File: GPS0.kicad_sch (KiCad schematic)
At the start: 12 parts, among them J2 GPS_ANT_0, U2 MAX-M10S-00B

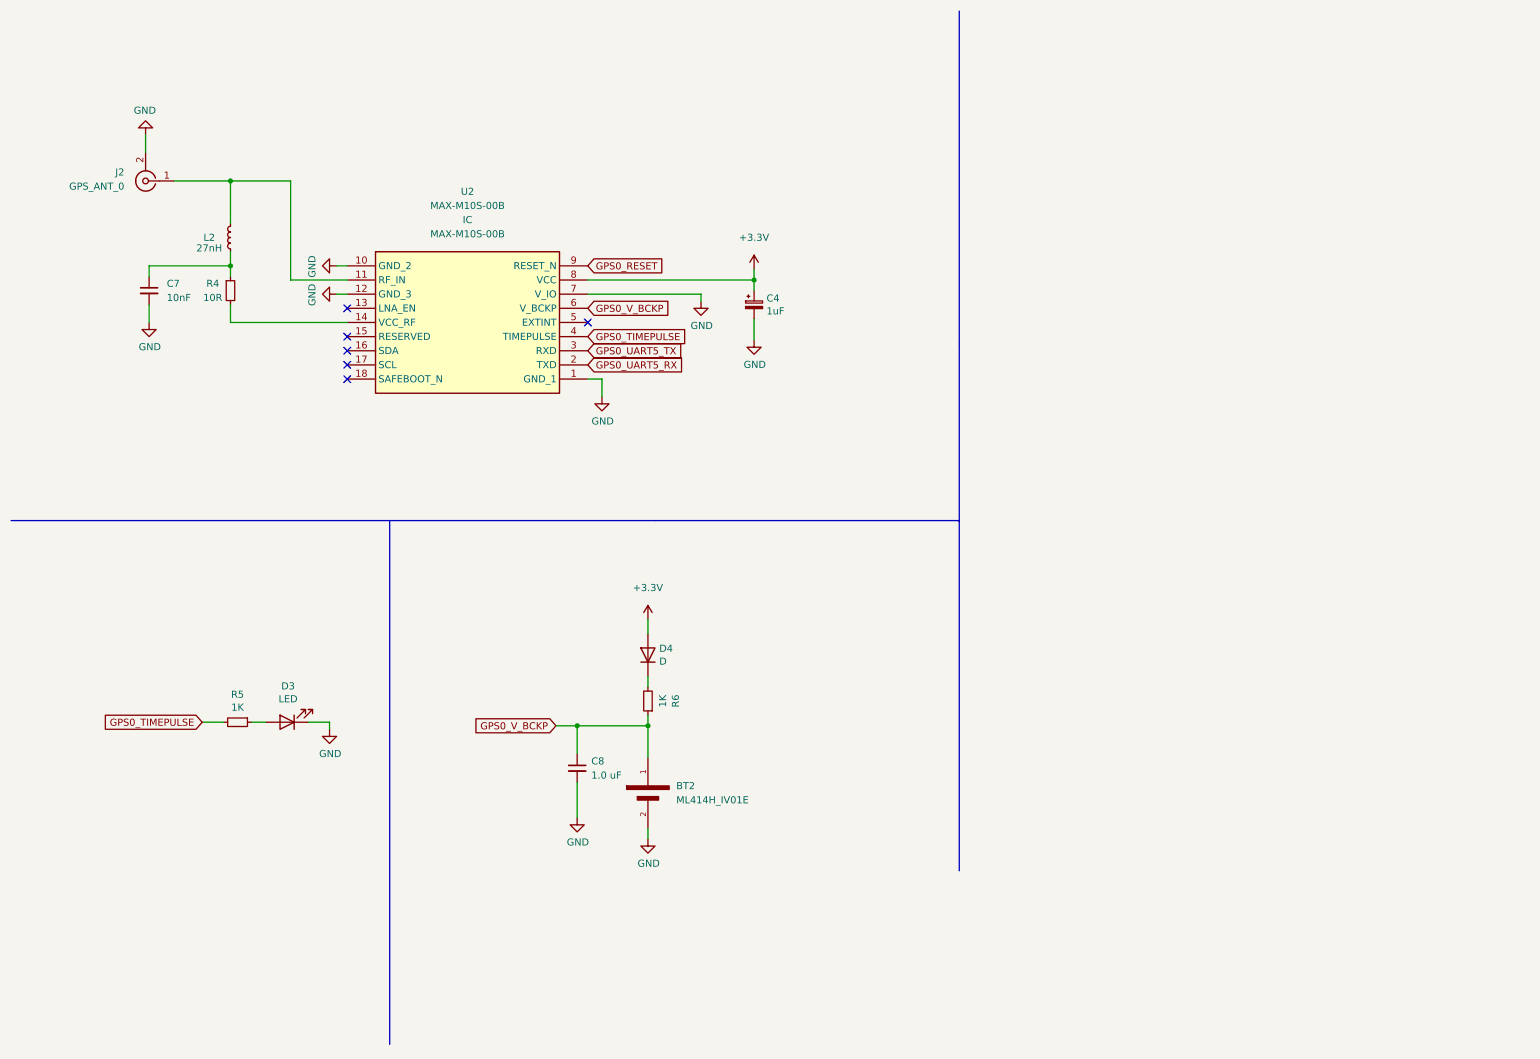
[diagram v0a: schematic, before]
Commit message: Last commit
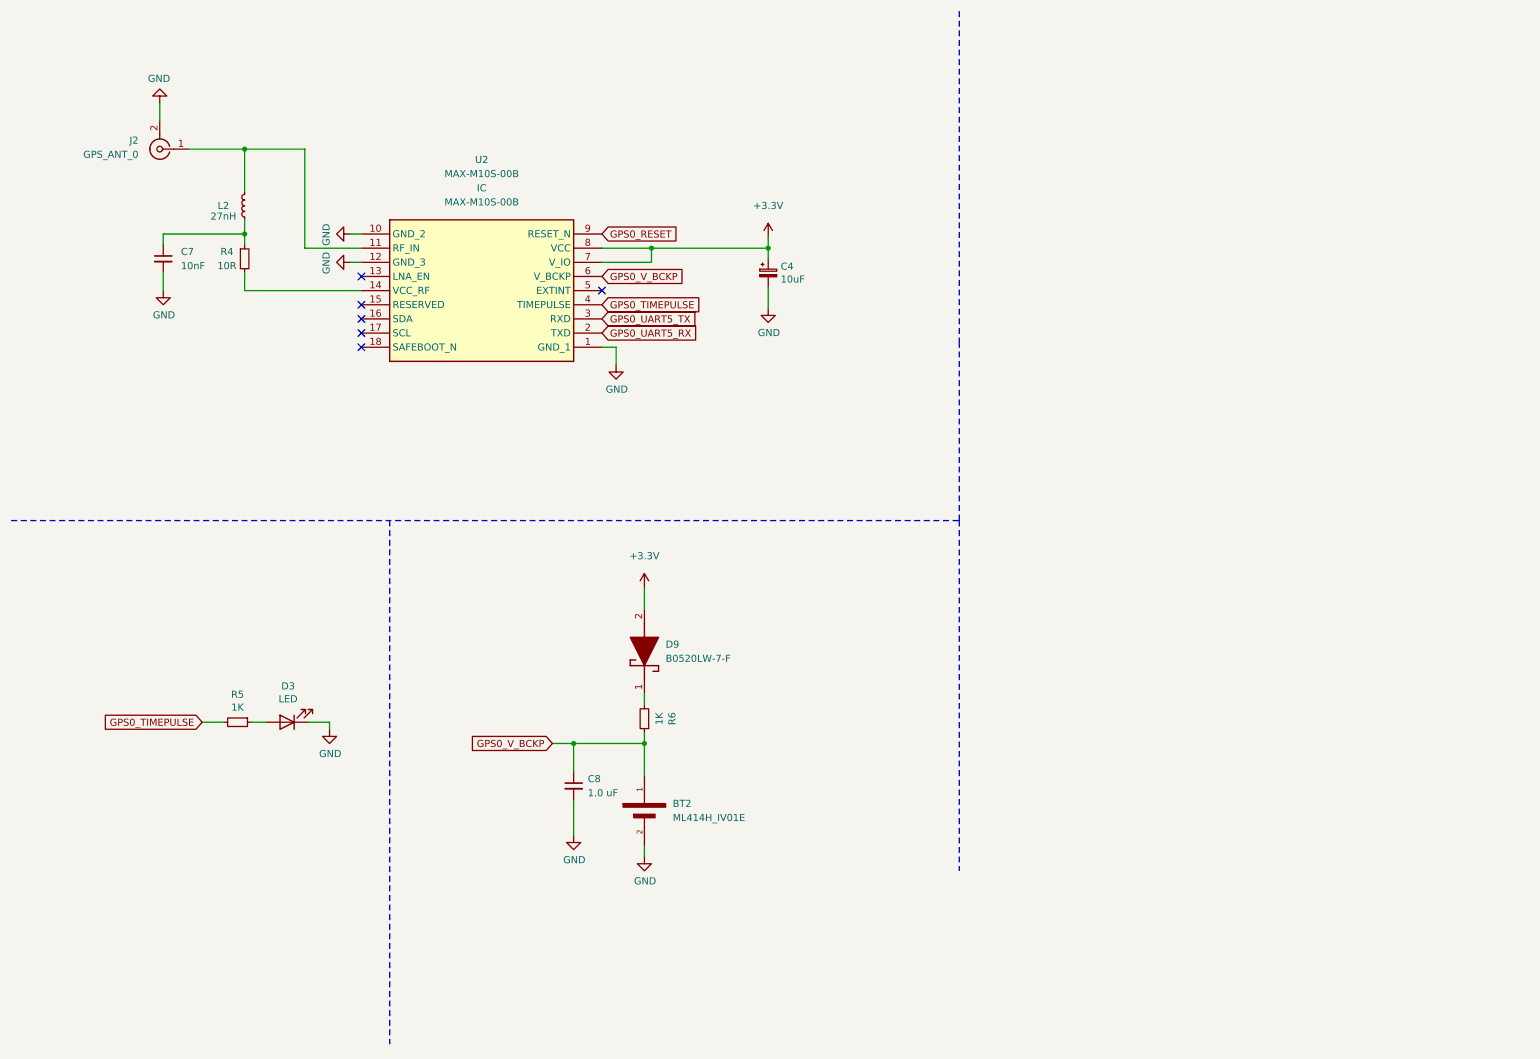
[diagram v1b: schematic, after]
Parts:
- removed D4: D, Diode_SMD:D_1206_3216Metric_Pad1.42x1.75mm_HandSolder, symbol Device:D
- added D9: B0520LW-7-F, B0520LW-7-F:SOD3716X145N, symbol B0520LW-7-F:B0520LW-7-F
- C4: value 1uF -> 10uF; footprint Capacitor_Tantalum_SMD:CP_EIA-3528-21_Kemet-B_Pad1.50x2.35mm_HandSolder -> Capacitor_SMD:C_1210_3225Metric
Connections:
- net +3.3V: now also U2.7 (V_IO), D9.2 (A)
- net GND: no longer U2.7 (V_IO)
- net at R6.2: now also D9.1 (K)
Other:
- moved on the sheet: BT2, C4, C7, C8, J2, L2, R4, R6, U2

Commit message: Second commit
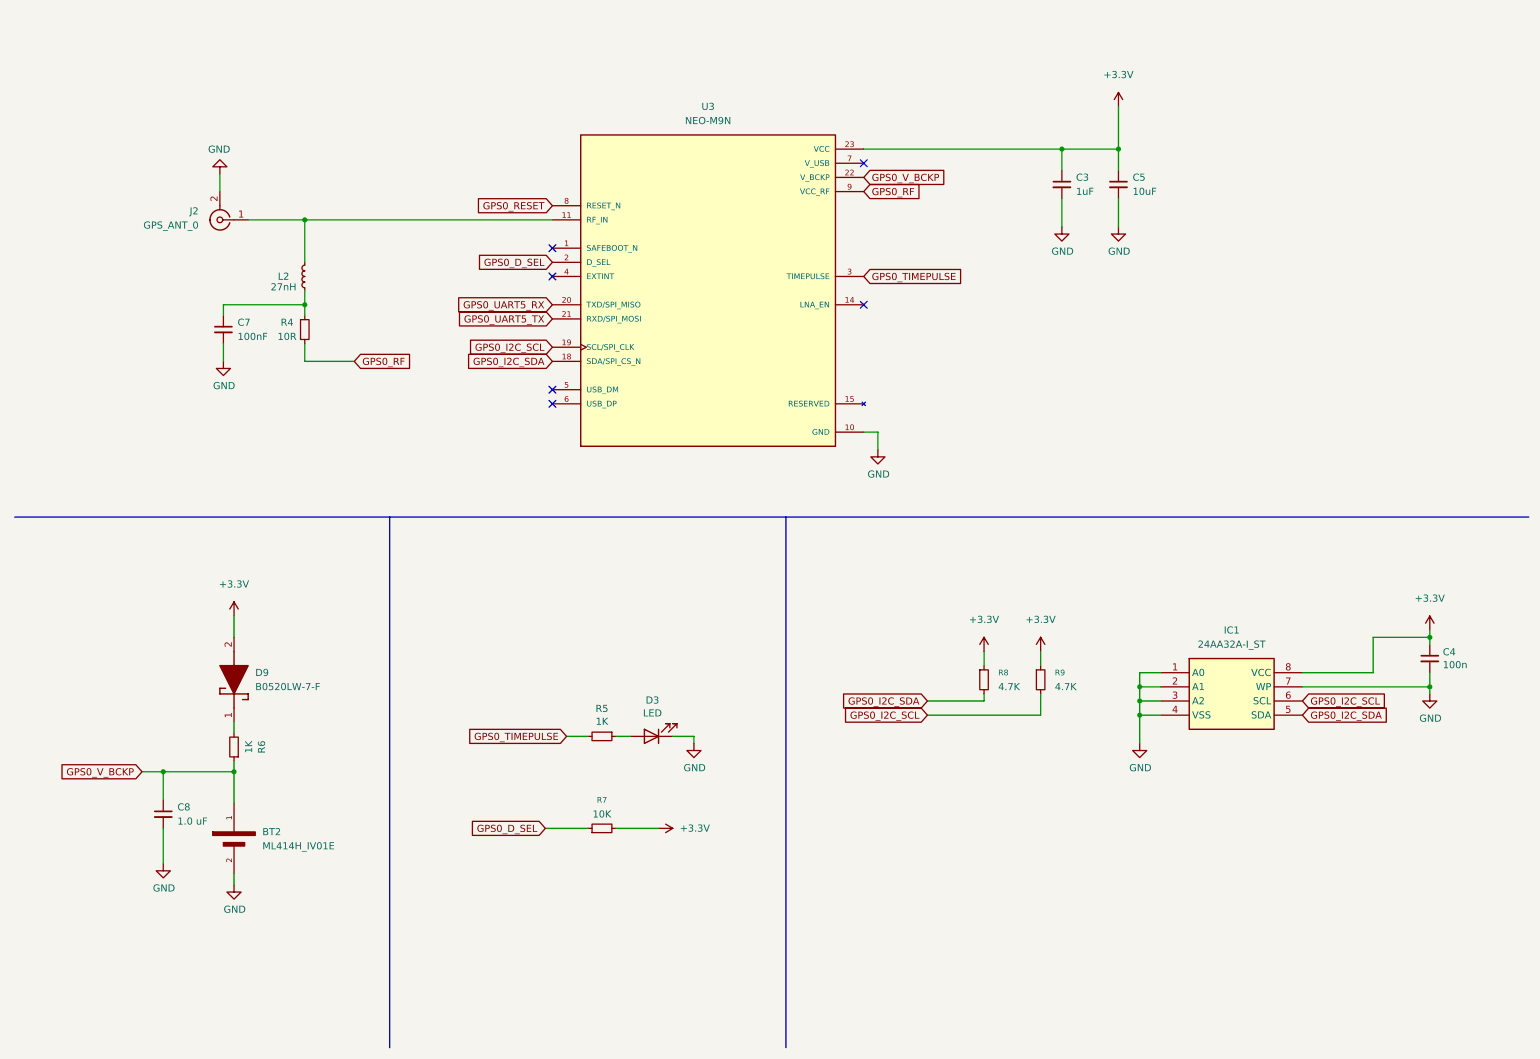
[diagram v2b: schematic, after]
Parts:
- removed C4: 10uF, Capacitor_SMD:C_1210_3225Metric, symbol Device:CP_Small
- removed U2: MAX-M10S-00B, MAX-M10S-00B:MAXM10S00B, symbol MAX-M10S-00B:MAX-M10S-00B
- added C3: 1uF, Capacitor_SMD:C_1210_3225Metric, symbol Device:C_Small
- added C4: 100n, Capacitor_SMD:C_0402_1005Metric, symbol Device:C_Small
- added C5: 10uF, Capacitor_SMD:C_1210_3225Metric, symbol Device:C_Small
- added IC1: 24AA32A-I_ST, 24AA32A-I_ST:SOP65P640X120-8N, symbol 24AA32A-I_ST:24AA32A-I_ST
- added R7: 10K, Resistor_SMD:R_0402_1005Metric, symbol Device:R_Small
- added R8, R9: 4.7K, Resistor_SMD:R_0402_1005Metric, symbol Device:R_Small
- added U3: NEO-M9N, NEO-M9N:XCVR_NEO-M9N, symbol NEO-M9N:NEO-M9N
- BT2: footprint ML414H_IV01E:SEIKO_ML414H_IV01E -> ML414H IV01E:SEIKO_ML414H_IV01E
- C7: value 10nF -> 100nF
- J2: footprint Connector_Coaxial:SMA_Samtec_SMA-J-P-X-ST-EM1_EdgeMount -> Connector_Coaxial:SMA_Samtec_SMA-J-P-H-ST-EM1_EdgeMount
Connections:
- net +3.3V: now also C3.1, C4.1, C5.1, IC1.8 (VCC), R7.2, R8.1, R9.1, U3.23 (VCC)
- net GND: now also C3.2, C4.2, C5.2, IC1.1 (A0), IC1.2 (A1), IC1.3 (A2), IC1.4 (VSS), IC1.7 (WP), U3.10 (GND), U3.12 (GND), U3.13 (GND), U3.24 (GND)
- net GPS0_RESET: now also U3.8 (RESET_N)
- net GPS0_TIMEPULSE: now also U3.3 (TIMEPULSE)
- net GPS0_UART5_RX: now also U3.20 (TXD/SPI_MISO)
- net GPS0_UART5_TX: now also U3.21 (RXD/SPI_MOSI)
- net GPS0_V_BCKP: now also U3.22 (V_BCKP)
- net at J2.1 (In), L2.2: now also U3.11 (RF_IN)
- net GPS0_RF: now reaches R4.2
- net GPS0_RF: now also U3.9 (VCC_RF)
- new net: U3.15 (RESERVED), U3.16 (RESERVED), U3.17 (RESERVED)
- new net GPS0_D_SEL: R7.1, U3.2 (D_SEL)
- new net GPS0_I2C_SCL: IC1.6 (SCL), R9.2, U3.19 (SCL/SPI_CLK)
- new net GPS0_I2C_SDA: IC1.5 (SDA), R8.2, U3.18 (SDA/SPI_CS_N)
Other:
- moved on the sheet: BT2, C7, C8, D3, D9, J2, L2, R4, R5, R6
